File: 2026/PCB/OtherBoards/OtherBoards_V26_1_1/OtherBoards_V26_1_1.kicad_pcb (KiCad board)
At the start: 2 copper layers, 50 x 22 mm, 14 parts, among them J1 Conn_01x03

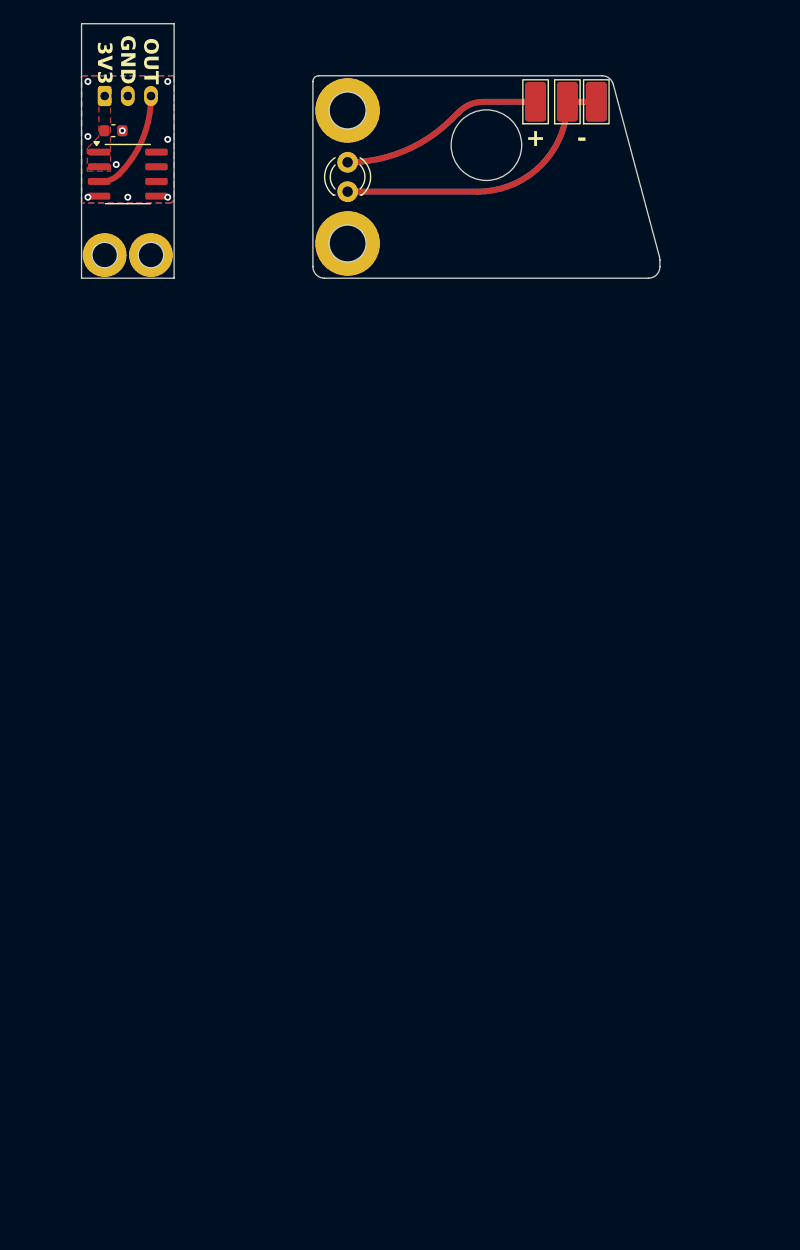
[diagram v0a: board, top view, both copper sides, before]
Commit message: 製造ファイル生成
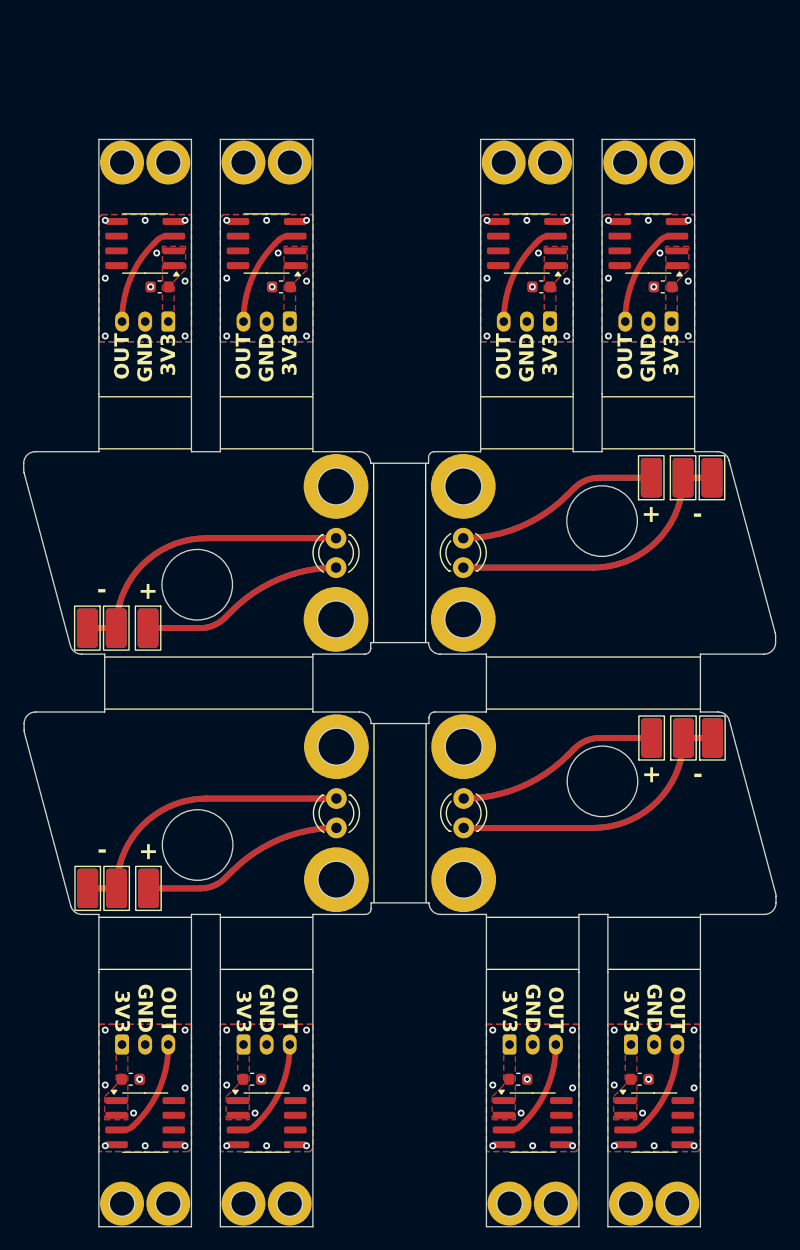
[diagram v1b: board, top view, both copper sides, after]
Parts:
- added C1: 0.1uf, Capacitor_SMD:C_0603_1608Metric, F.Cu at (42.2, 50.8)
- added C1: 0.1uf, Capacitor_SMD:C_0603_1608Metric, F.Cu at (75.2, 50.8)
- added C1: 0.1uf, Capacitor_SMD:C_0603_1608Metric, F.Cu at (62.8, 119.2)
- added C1: 0.1uf, Capacitor_SMD:C_0603_1608Metric, F.Cu at (64.8, 50.8)
- added C1: 0.1uf, Capacitor_SMD:C_0603_1608Metric, F.Cu at (39.8, 119.2)
- added C1: 0.1uf, Capacitor_SMD:C_0603_1608Metric, F.Cu at (31.8, 50.8)
- added C1: 0.1uf, Capacitor_SMD:C_0603_1608Metric, F.Cu at (29.2, 119.2)
- added D1: LED, 0-MyLibrary:LED_3mm_TopBottom, F.Cu at (58.0, 73.8)
- added D1: LED, 0-MyLibrary:LED_3mm_TopBottom, F.Cu at (47.0, 73.7)
- added D1: LED, 0-MyLibrary:LED_3mm_TopBottom, F.Cu at (47.0, 96.2)
- added H1: MountingHole, MountingHole:MountingHole_3.2mm_M3_DIN965_Pad, F.Cu at (47.0, 68.0)
- added H1: MountingHole, MountingHole:MountingHole_3.2mm_M3_DIN965_Pad, F.Cu at (47.0, 90.5)
- added H1: MountingHole, MountingHole:MountingHole_3.2mm_M3_DIN965_Pad, F.Cu at (58.0, 79.5)
- added H2: MountingHole, MountingHole:MountingHole_3.2mm_M3_DIN965_Pad, F.Cu at (58.0, 68.0)
- added H2: MountingHole, MountingHole:MountingHole_3.2mm_M3_DIN965_Pad, F.Cu at (47.0, 79.5)
- added H2: MountingHole, MountingHole:MountingHole_3.2mm_M3_DIN965_Pad, F.Cu at (47.0, 102.0)
- added H3: MountingHole, MountingHole:MountingHole_2.2mm_M2_DIN965_Pad, F.Cu at (39.0, 130.0)
- added H3: MountingHole, MountingHole:MountingHole_2.2mm_M2_DIN965_Pad, F.Cu at (76.0, 40.0)
- added H3: MountingHole, MountingHole:MountingHole_2.2mm_M2_DIN965_Pad, F.Cu at (28.5, 130.0)
- added H3: MountingHole, MountingHole:MountingHole_2.2mm_M2_DIN965_Pad, F.Cu at (65.5, 40.0)
- added H3: MountingHole, MountingHole:MountingHole_2.2mm_M2_DIN965_Pad, F.Cu at (43.0, 40.0)
- added H3: MountingHole, MountingHole:MountingHole_2.2mm_M2_DIN965_Pad, F.Cu at (32.5, 40.0)
- added H3: MountingHole, MountingHole:MountingHole_2.2mm_M2_DIN965_Pad, F.Cu at (62.0, 130.0)
- added H4: MountingHole, MountingHole:MountingHole_2.2mm_M2_DIN965_Pad, F.Cu at (32.5, 130.0)
- added H4: MountingHole, MountingHole:MountingHole_2.2mm_M2_DIN965_Pad, F.Cu at (72.0, 40.0)
- added H4: MountingHole, MountingHole:MountingHole_2.2mm_M2_DIN965_Pad, F.Cu at (39.0, 40.0)
- added H4: MountingHole, MountingHole:MountingHole_2.2mm_M2_DIN965_Pad, F.Cu at (43.0, 130.0)
- added H4: MountingHole, MountingHole:MountingHole_2.2mm_M2_DIN965_Pad, F.Cu at (28.5, 40.0)
- added H4: MountingHole, MountingHole:MountingHole_2.2mm_M2_DIN965_Pad, F.Cu at (66.0, 130.0)
- added H4: MountingHole, MountingHole:MountingHole_2.2mm_M2_DIN965_Pad, F.Cu at (61.5, 40.0)
- added J1: Conn_01x03, Connector_JST:JST_PH_S3B-PH-K_1x03_P2.00mm_Horizontal, B.Cu at (28.5, 116.2)
- added J1: Conn_01x03, Connector_JST:JST_PH_S3B-PH-K_1x03_P2.00mm_Horizontal, B.Cu at (65.5, 53.8)
- added J1: Conn_01x03, Connector_JST:JST_PH_S3B-PH-K_1x03_P2.00mm_Horizontal, B.Cu at (32.5, 53.8)
- added J1: Conn_01x03, Connector_JST:JST_PH_S3B-PH-K_1x03_P2.00mm_Horizontal, B.Cu at (76.0, 53.8)
- added J1: Conn_01x03, Connector_JST:JST_PH_S3B-PH-K_1x03_P2.00mm_Horizontal, B.Cu at (43.0, 53.8)
- added J1: Conn_01x03, Connector_JST:JST_PH_S3B-PH-K_1x03_P2.00mm_Horizontal, B.Cu at (39.0, 116.2)
- added J1: Conn_01x03, Connector_JST:JST_PH_S3B-PH-K_1x03_P2.00mm_Horizontal, B.Cu at (62.0, 116.2)
- added TP1: TestPoint, TestPoint:TestPoint_Keystone_5015_Micro_Mini, F.Cu at (28.0, 80.2)
- added TP1: TestPoint, TestPoint:TestPoint_Keystone_5015_Micro_Mini, F.Cu at (77.0, 67.3)
- added TP1: TestPoint, TestPoint:TestPoint_Keystone_5015_Micro_Mini, F.Cu at (28.0, 102.7)
- added TP2: TestPoint, TestPoint:TestPoint_Keystone_5015_Micro_Mini, F.Cu at (79.5, 67.3)
- added TP2: TestPoint, TestPoint:TestPoint_Keystone_5015_Micro_Mini, F.Cu at (25.5, 80.2)
- added TP2: TestPoint, TestPoint:TestPoint_Keystone_5015_Micro_Mini, F.Cu at (25.5, 102.7)
- added TP3: TestPoint, TestPoint:TestPoint_Keystone_5015_Micro_Mini, F.Cu at (74.2, 67.3)
- added TP3: TestPoint, TestPoint:TestPoint_Keystone_5015_Micro_Mini, F.Cu at (30.8, 80.2)
- added TP3: TestPoint, TestPoint:TestPoint_Keystone_5015_Micro_Mini, F.Cu at (30.8, 102.7)
- added TP4: TestPoint, TestPoint:TestPoint_Keystone_5015_Micro_Mini, B.Cu at (28.0, 80.2)
- added TP4: TestPoint, TestPoint:TestPoint_Keystone_5015_Micro_Mini, B.Cu at (28.0, 102.7)
- added TP4: TestPoint, TestPoint:TestPoint_Keystone_5015_Micro_Mini, B.Cu at (77.0, 67.3)
- added TP5: TestPoint, TestPoint:TestPoint_Keystone_5015_Micro_Mini, B.Cu at (25.5, 102.7)
- added TP5: TestPoint, TestPoint:TestPoint_Keystone_5015_Micro_Mini, B.Cu at (25.5, 80.2)
- added TP5: TestPoint, TestPoint:TestPoint_Keystone_5015_Micro_Mini, B.Cu at (79.5, 67.3)
- added TP6: TestPoint, TestPoint:TestPoint_Keystone_5015_Micro_Mini, B.Cu at (74.2, 67.3)
- added TP6: TestPoint, TestPoint:TestPoint_Keystone_5015_Micro_Mini, B.Cu at (30.8, 80.2)
- added TP6: TestPoint, TestPoint:TestPoint_Keystone_5015_Micro_Mini, B.Cu at (30.8, 102.7)
- added U1: ~, Package_SO:SOIC-8_3.9x4.9mm_P1.27mm, F.Cu at (64.0, 123.0)
- added U1: ~, Package_SO:SOIC-8_3.9x4.9mm_P1.27mm, F.Cu at (30.5, 123.0)
- added U1: ~, Package_SO:SOIC-8_3.9x4.9mm_P1.27mm, F.Cu at (41.0, 47.0)
- added U1: ~, Package_SO:SOIC-8_3.9x4.9mm_P1.27mm, F.Cu at (63.5, 47.0)
- added U1: ~, Package_SO:SOIC-8_3.9x4.9mm_P1.27mm, F.Cu at (74.0, 47.0)
- added U1: ~, Package_SO:SOIC-8_3.9x4.9mm_P1.27mm, F.Cu at (41.0, 123.0)
- added U1: ~, Package_SO:SOIC-8_3.9x4.9mm_P1.27mm, F.Cu at (30.5, 47.0)
- moved C1 93.8 mm to (73.2, 119.2)
- moved H3 93.8 mm to (72.5, 130.0)
- moved H4 93.8 mm to (76.5, 130.0)
- moved J1 93.8 mm to (72.5, 116.2)
- moved U1 93.8 mm to (74.5, 123.0)
- moved D1 55.9 mm to (58.0, 96.3)
- moved H1 55.9 mm to (58.0, 102.0)
- moved H2 55.9 mm to (58.0, 90.5)
- moved TP1 55.9 mm to (77.0, 89.8)
- moved TP2 55.9 mm to (79.5, 89.8)
- moved TP3 55.9 mm to (74.3, 89.8)
- moved TP4 55.9 mm to (77.0, 89.8)
- moved TP5 55.9 mm to (79.5, 89.8)
- moved TP6 55.9 mm to (74.3, 89.8)
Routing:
- net Net-(D1-K): track 51.2 -> 205.0 mm
- net Net-(D1-A): track 35.3 -> 141.3 mm
- net OUT: track 9.32 -> 75.0 mm
- net GND: vias 9 -> 72
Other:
- board size 50 x 22 mm -> 65 x 94 mm
